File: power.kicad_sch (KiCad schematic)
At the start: 49 parts, among them J1 Battery 1, J7 Battery 2, J8 USB, U1 AMS1117-3.3, U5 TPS56A37RPAR, U6 TPS56A37RPAR

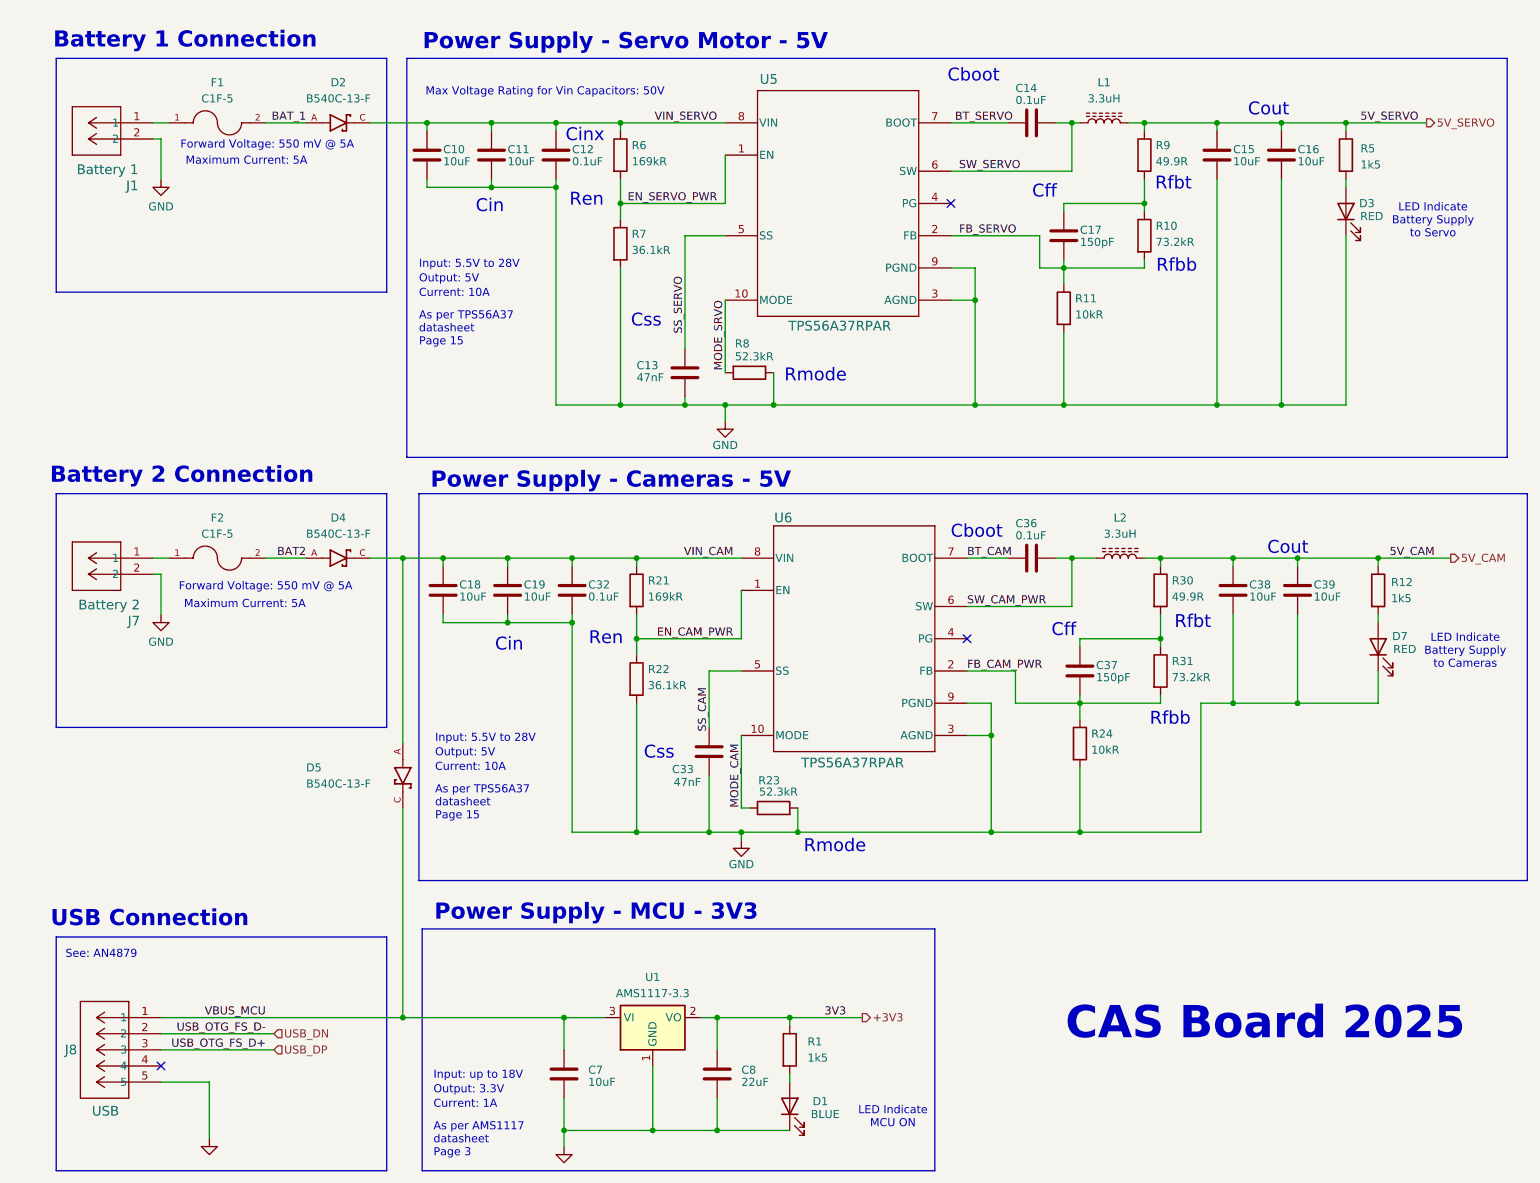
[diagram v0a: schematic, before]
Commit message: Sync
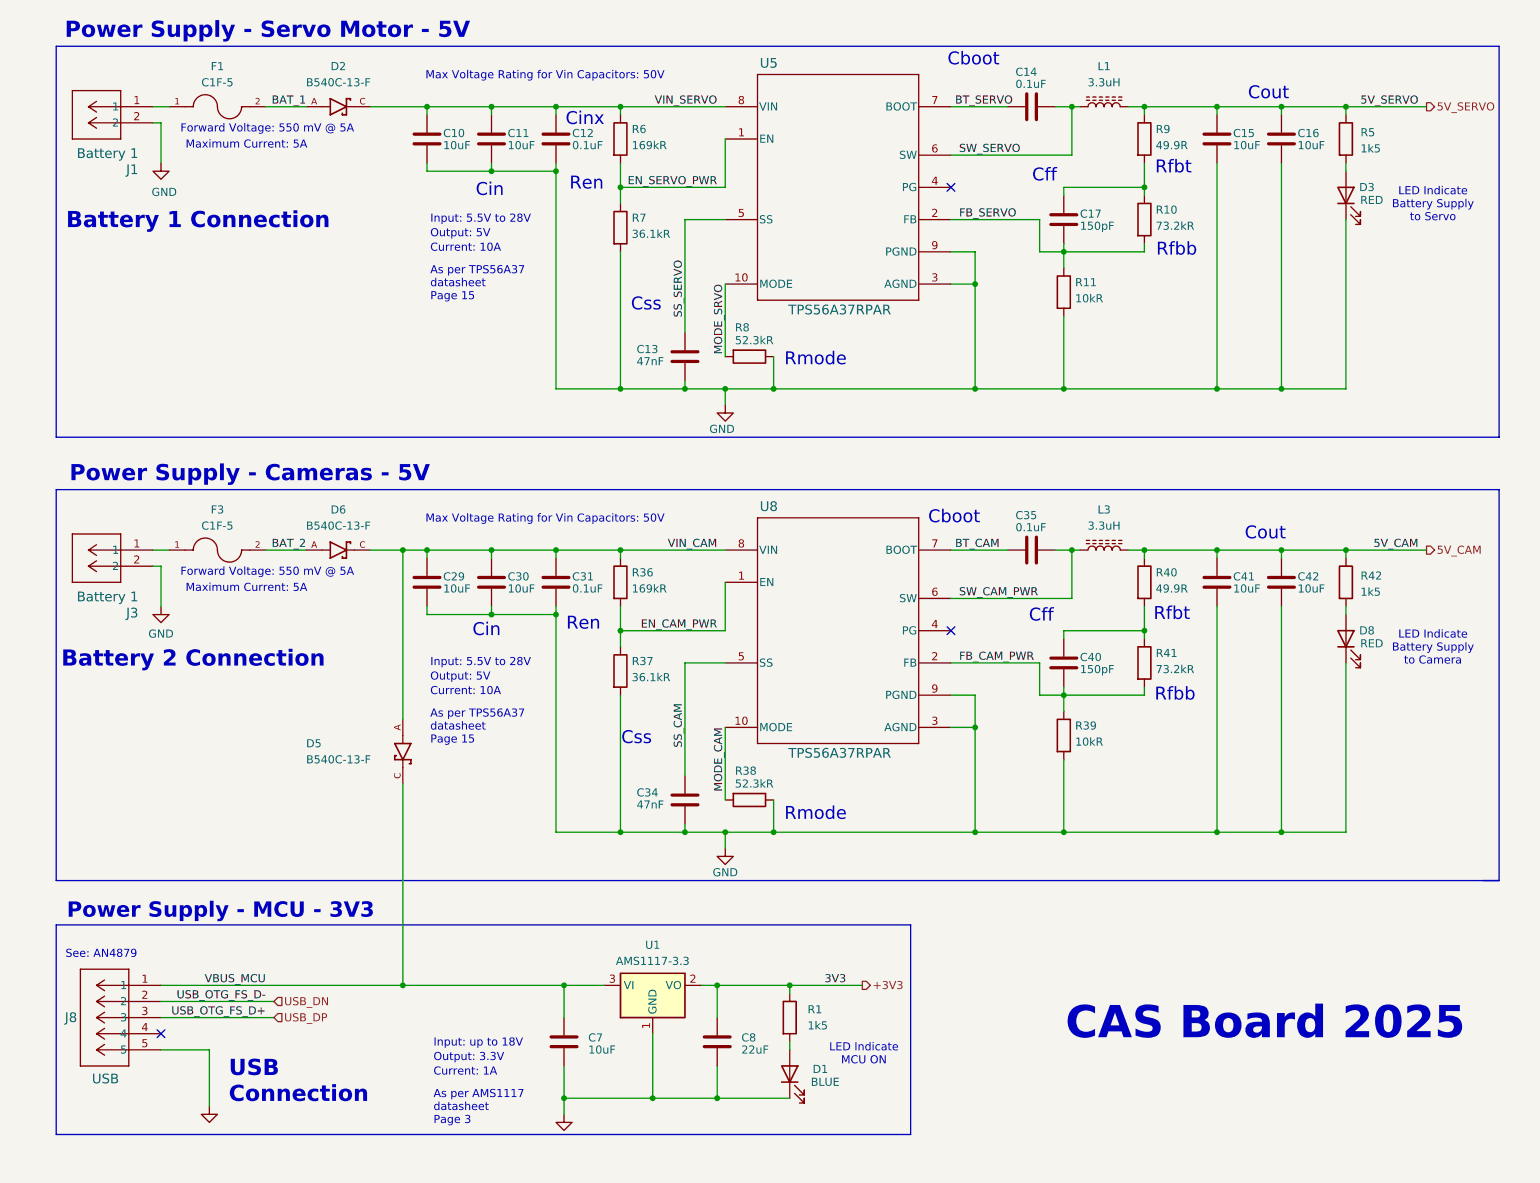
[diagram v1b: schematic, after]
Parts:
- removed C18, C19, C38, C39: 10uF, Capacitor_SMD:C_0805_2012Metric, symbol Device:C
- removed C32, C36: 0.1uF, Capacitor_SMD:C_0805_2012Metric, symbol Device:C
- removed C33: 47nF, Capacitor_SMD:C_0805_2012Metric, symbol Device:C
- removed C37: 150pF, Capacitor_SMD:C_0805_2012Metric, symbol Device:C
- removed D4: B540C-13-F, B540C_13_F:DIOM6959X245N, symbol B540C-13-F:B540C-13-F
- removed D7: RED, LED_SMD:LED_0805_2012Metric, symbol Device:LED
- removed F2: C1F-5, C1F_5:FUSC3215X83N, symbol C1F-5:C1F-5
- removed J7: Battery 2, 39-28-1023:CONN_SD-5566-002_02_MOL, symbol 39-28-1023:39281023
- removed L2: 3.3uH, Inductor_SMD:L_0805_2012Metric_Pad1.05x1.20mm_HandSolder, symbol Device:L_Ferrite
- removed R12: 1k5, Resistor_SMD:R_0805_2012Metric_Pad1.20x1.40mm_HandSolder, symbol Device:R
- removed R21: 169kR, Capacitor_SMD:C_0805_2012Metric, symbol Device:R
- removed R22: 36.1kR, Capacitor_SMD:C_0805_2012Metric, symbol Device:R
- removed R23: 52.3kR, Capacitor_SMD:C_0805_2012Metric, symbol Device:R
- removed R24: 10kR, Capacitor_SMD:C_0805_2012Metric, symbol Device:R
- removed R30: 49.9R, Capacitor_SMD:C_0805_2012Metric, symbol Device:R
- removed R31: 73.2kR, Capacitor_SMD:C_0805_2012Metric, symbol Device:R
- removed U6: TPS56A37RPAR, RPA0010A-MFG, symbol TPS56A37RPAR:TPS56A37RPAR
- added C29, C30: 10uF, Capacitor_SMD:C_1206_3216Metric, symbol Device:C
- added C31, C35: 0.1uF, Capacitor_SMD:C_0805_2012Metric, symbol Device:C
- added C34: 47nF, Capacitor_SMD:C_0805_2012Metric, symbol Device:C
- added C40: 150pF, Capacitor_SMD:C_0805_2012Metric, symbol Device:C
- added C41, C42: 10uF, Capacitor_SMD:C_1210_3225Metric, symbol Device:C
- added D6: B540C-13-F, B540C_13_F:DIOM6959X245N, symbol B540C-13-F:B540C-13-F
- added D8: RED, LED_SMD:LED_0805_2012Metric, symbol Device:LED
- added F3: C1F-5, C1F_5:FUSC3215X83N, symbol C1F-5:C1F-5
- added J3: Battery 1, 1724480002:MOLEX_1724480002, symbol 39-28-1023:39281023
- added L3: 3.3uH, 74438357033:WE-MAPI_4030, symbol Device:L_Ferrite
- added R36: 169kR, Capacitor_SMD:C_0805_2012Metric, symbol Device:R
- added R37: 36.1kR, Capacitor_SMD:C_0805_2012Metric, symbol Device:R
- added R38: 52.3kR, Capacitor_SMD:C_0805_2012Metric, symbol Device:R
- added R39: 10kR, Capacitor_SMD:C_0805_2012Metric, symbol Device:R
- added R40: 49.9R, Capacitor_SMD:C_0805_2012Metric, symbol Device:R
- added R41: 73.2kR, Capacitor_SMD:C_0805_2012Metric, symbol Device:R
- added R42: 1k5, Capacitor_SMD:C_0805_2012Metric, symbol Device:R
- added U8: TPS56A37RPAR, RPA0010A-MFG, symbol TPS56A37RPAR:TPS56A37RPAR
- J1: footprint 39-28-1023:CONN_SD-5566-002_02_MOL -> 1724480002:MOLEX_1724480002
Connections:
- net 5V_CAM: now also C41.1, C42.1, L3.2, R40.1, R42.1
- net BT_CAM: now also C35.1, U8.7 (BOOT)
- net EN_CAM_PWR: now also R36.2, R37.1, U8.1 (EN)
- net FB_CAM_PWR: now also C40.2, R39.1, R41.2, U8.2 (FB)
- net GND: now also C29.2, C30.2, C31.2, C34.2, C41.2, C42.2, D8.1 (K), J3.2, R37.2, R38.1, R39.2, U8.3 (AGND), U8.9 (PGND)
- net MODE_CAM: now also R38.2, U8.10 (MODE)
- net SS_CAM: now also C34.1, U8.5 (SS)
- net SW_CAM_PWR: now also C35.2, L3.1, U8.6 (SW)
- net VIN_CAM: now also C29.1, C30.1, C31.1, D6.C, R36.1, U8.8 (VIN)
- new net: C40.1, R40.2, R41.1
- new net: F3.1, J3.1
- new net: D8.2 (A), R42.2
- new net BAT_2: D6.A, F3.2
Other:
- note added: "LED Indicate Battery Supply to Camera"
- note removed: "LED Indicate Battery Supply to Cameras"
- moved on the sheet: C10, C11, C12, C13, C14, C15, C16, C17, C7, C8, D1, D2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
